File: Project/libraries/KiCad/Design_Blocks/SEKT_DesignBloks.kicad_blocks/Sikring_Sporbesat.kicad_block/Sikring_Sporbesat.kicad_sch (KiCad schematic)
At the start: 18 parts, among them J1 Screw_Terminal_01x02, J2 Screw_Terminal_01x02, J3 Conn_01x05_Socket, Q1 BC857, U1 PC847

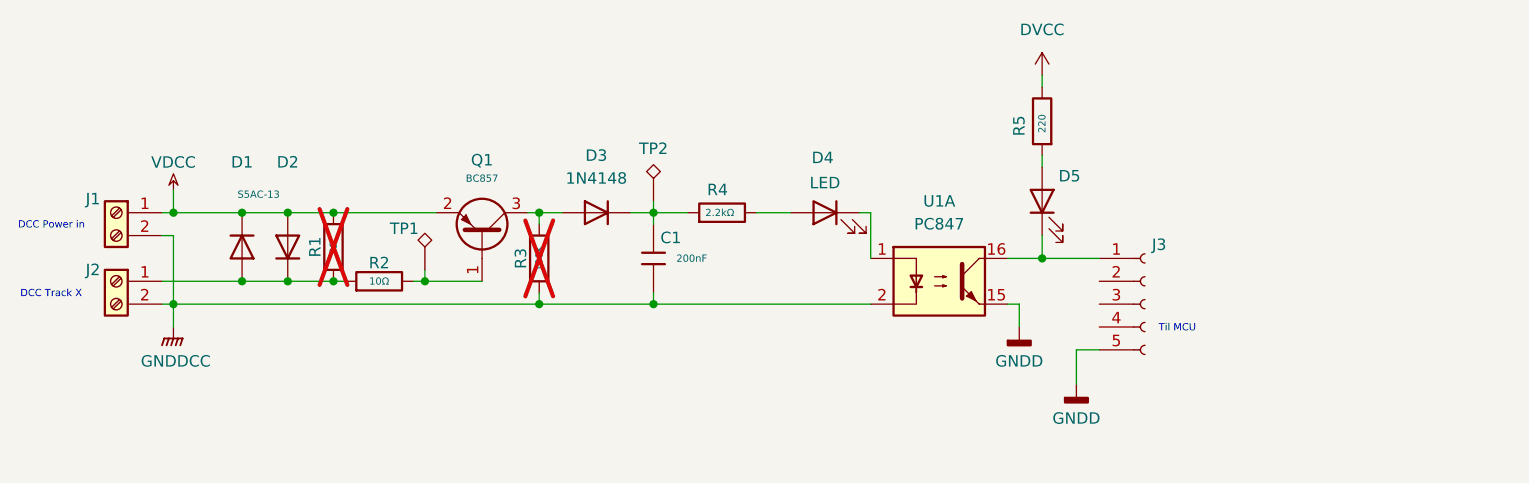
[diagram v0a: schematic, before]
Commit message: Beskrivelse af functionen af Sporbesat detektor
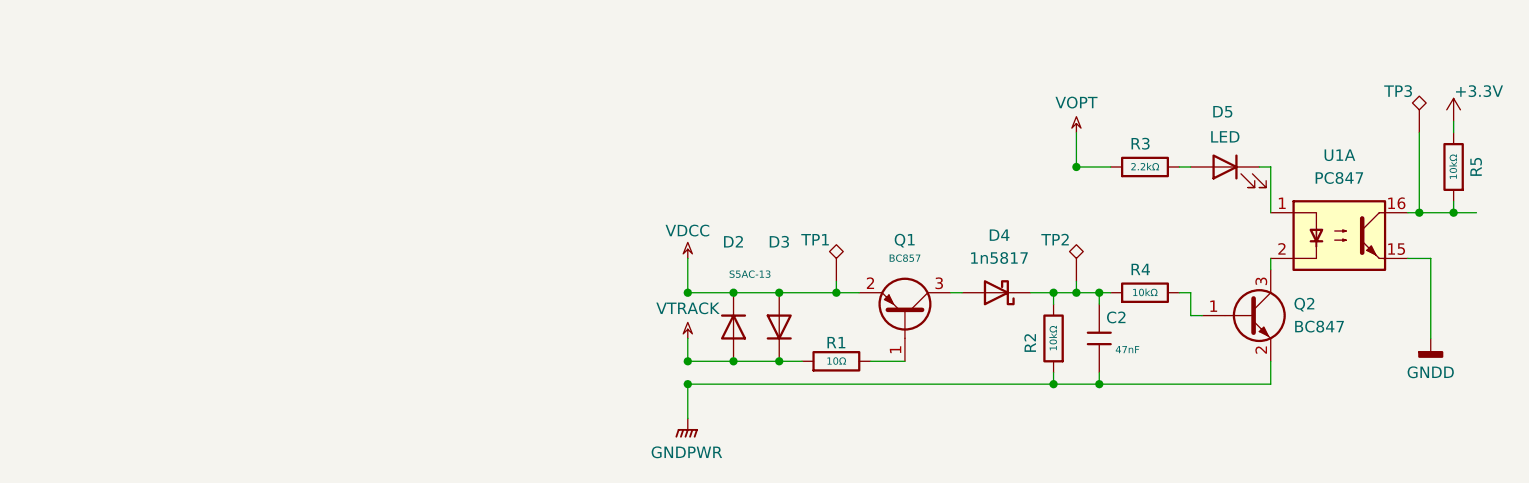
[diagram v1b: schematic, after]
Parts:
- removed D3: 1N4148, Diode_THT:D_DO-35_SOD27_P7.62mm_Horizontal, symbol Diode:1N4148
- removed D5: LED, LED_SMD:LED_0805_2012Metric, symbol Device:LED
- removed J1: Screw_Terminal_01x02, Package_SON:WSON-8-1EP_6x5mm_P1.27mm_EP3.4x4mm, symbol Connector:Screw_Terminal_01x02
- removed J2: Screw_Terminal_01x02, symbol Connector:Screw_Terminal_01x02
- removed J3: Conn_01x05_Socket, symbol Connector:Conn_01x05_Socket
- removed R1: ?Ω, PCM_JLCPCB:R_0805, symbol PCM_JLCPCB-Resistors:0805,1.8kΩ
- removed R3: 100K, PCM_JLCPCB:R_0805, symbol PCM_JLCPCB-Resistors:0805,1.8kΩ
- removed TP2: U1A_Collector, TestPoint:TestPoint_Loop_D2.60mm_Drill1.4mm_Beaded, symbol Connector:TestPoint_Alt
- added D4: 1n5817, symbol Device:D_Schottky
- added Q2: BC847, Package_TO_SOT_SMD:SOT-23, symbol Transistor_BJT:BC847
- added R2, R4: 10kΩ, PCM_JLCPCB:R_0805, symbol PCM_JLCPCB-Resistors:0805,1.8kΩ
- added TP1, TP3: Q1_Basic, TestPoint:TestPoint_Loop_D2.60mm_Drill1.4mm_Beaded, symbol Connector:TestPoint_Alt
- C2: renamed from C1; value 200nF -> 47nF
- R5: value 220 -> 10kΩ
- renumbered D1 to D2, D2 to D3, D4 to D5, R2 to R1, R4 to R3, TP1 to TP2
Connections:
- net VDCC: now also TP1.1
- net at Q1.3 (C): now also D4.2 (A)
- net at Q1.1 (B), R1.2: no longer TP2.1
- net at U1.16: now also R5.1, TP3.1
- net at C2.1: now also TP2.1, D4.1 (K), R2.2, R4.1; no longer R3.1
- net VTRACK: now reaches D2.2 (A), D3.1 (K), R1.1
- net DVCC renamed +3.3V
- net GNDDCC: no longer names the net of U1.2
- net GNDDCC: now also Q2.3 (C); no longer C2.2
- new net: Q2.1 (B), R4.2
- new net GNDPWR: C2.2, Q2.2 (E), R2.1
- new net VOPT: R3.1
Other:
- note removed: "DCC Power in"
- note removed: "DCC Track X"
- note removed: "Til MCU"
- moved on the sheet: C2, D2, D3, D5, Q1, R1, R3, TP2, U1A
